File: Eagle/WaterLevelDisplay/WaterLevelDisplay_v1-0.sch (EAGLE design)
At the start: 17 parts, among them J12 POWER_JACKPTH_BREAD, J7 RJ45

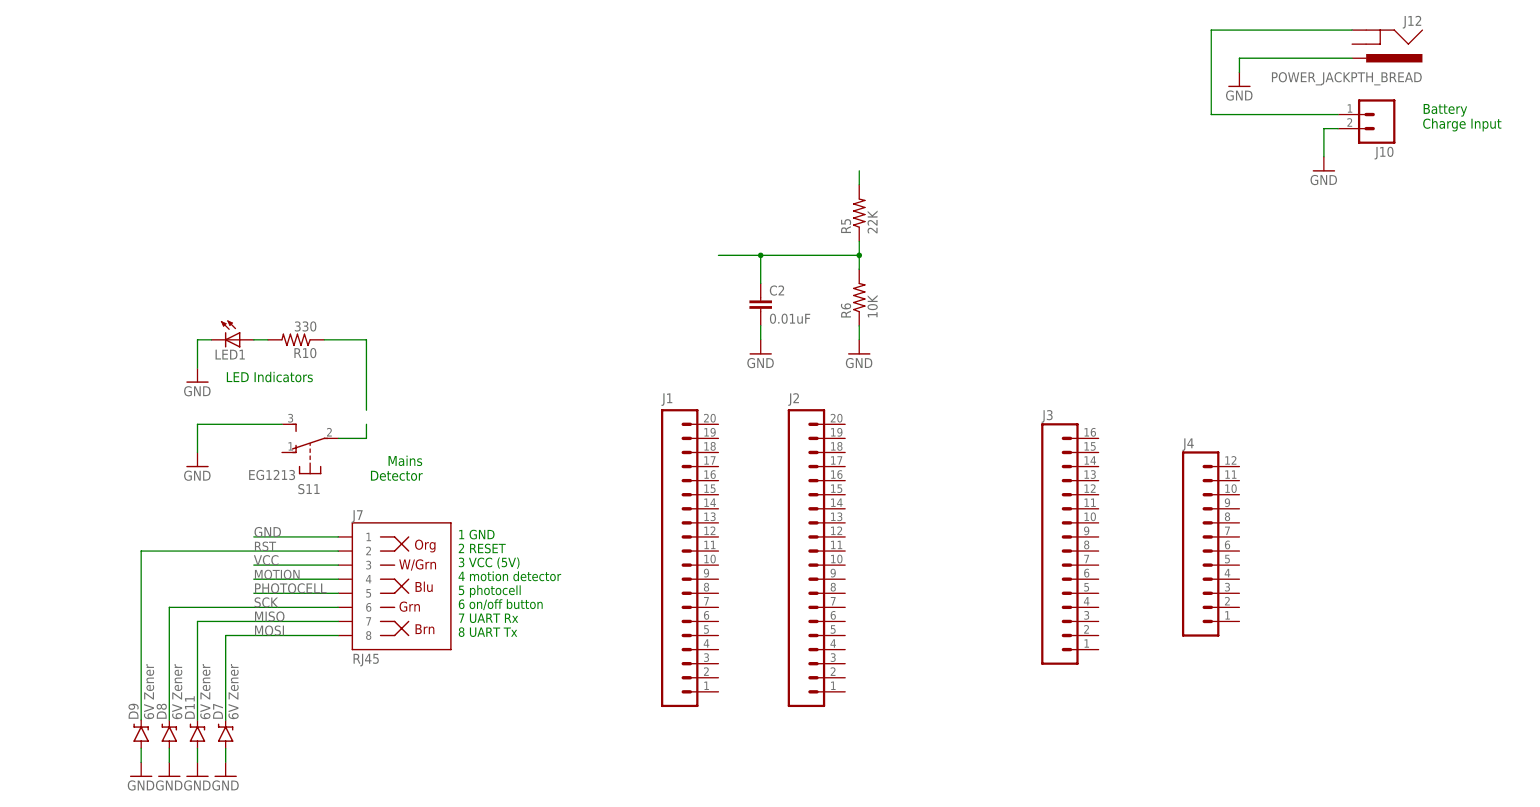
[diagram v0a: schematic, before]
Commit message: first round of layout
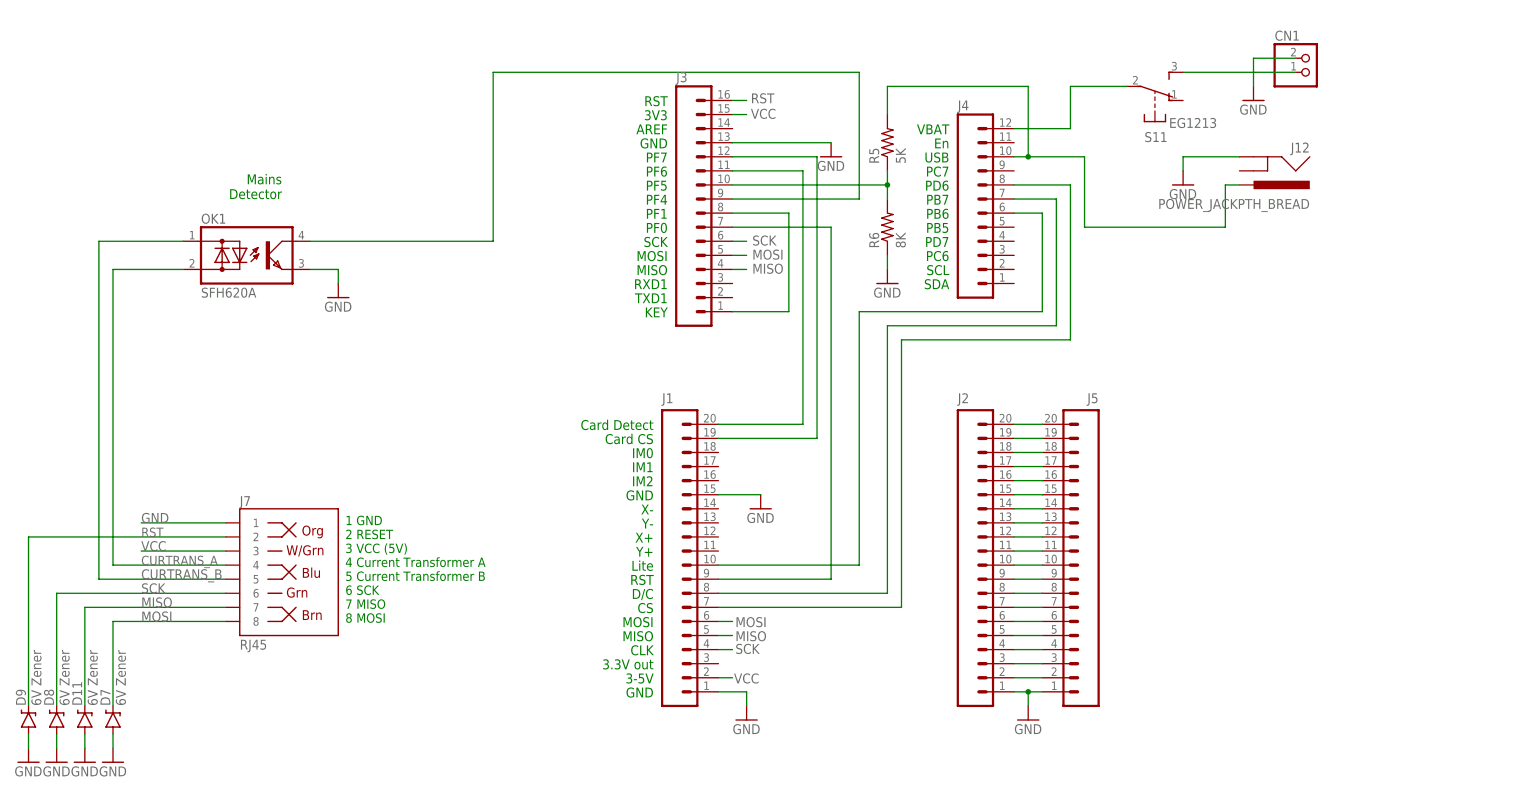
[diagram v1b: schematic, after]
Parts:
- removed C2: 0.01uF, SparkFun-Passives:CAPPTH1
- removed J10: (no value), SparkFun-Connectors:M02PTH
- removed LED1: (no value), adafruit:LED5MM
- removed R10: 330, resistor:R-US_0204/5
- added CN1: (no value), adafruit:JST_2PIN-SMT-RA
- added J5: (no value), SparkFun-Connectors:M20NOSILK
- added OK1: SFH620A, optocoupler:SFH620A
- R5: value 22K -> 5K
- R6: value 10K -> 8K
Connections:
- removed net MOTION: J7.4
- removed net N$6: C2.1, R5.1, R6.2
- removed net PHOTOCELL: J7.5
- new net CURTRANS_A: J7.4, OK1.AC2
- new net CURTRANS_B: J7.5, OK1.AC1
- new net N$10: J2.8, J5.8
- new net N$11: J2.9, J5.9
- new net N$12: J2.10, J5.10
- new net N$13: J2.11, J5.11
- new net N$14: J2.12, J5.12
- new net N$16: J2.13, J5.13
- new net N$19: J2.14, J5.14
- new net N$2: J2.2, J5.2
- new net N$20: J2.15, J5.15
- new net N$21: J2.16, J5.16
- new net N$22: J2.17, J5.17
- new net N$23: J2.18, J5.18
- new net N$24: J2.19, J5.19
- new net N$25: J2.20, J5.20
- new net N$27: J1.8, J4.7
- new net N$28: J1.19, J3.12
- new net N$29: J1.20, J3.11
- new net N$3: J2.3, J5.3
- new net N$30: J1.10, J4.6
- new net N$31: J3.9, OK1.C
- new net N$32: J1.7, J4.8
- new net N$33: J1.9, J3.7
- new net N$4: J2.4, J5.4
- new net N$5: J2.5, J5.5
- new net N$7: J2.6, J5.6
- new net N$8: J2.7, J5.7
- net GND: now also CN1.1, J1.1, J1.15, J12.GND, J2.1, J3.13, J5.1, OK1.E; no longer C2.2, J10.2, J12.PWR, LED1.C, S11.S
- net MISO: now also J1.5, J3.4
- net MOSI: now also J1.6, J3.5
- net N$1: now also CN1.2, S11.S; no longer LED1.A, R10.2
- net N$15: now also J3.1, J3.8; no longer R10.1
- net N$17: now also J12.PWR, J4.10, R5.2; no longer J10.1, J12.GND
- net N$18: now also J3.10, R5.1, R6.2; no longer R5.2
- net N$9: now also J4.12
- net RST: now also J3.16
- net SCK: now also J1.4, J3.6
- net VCC: now also J1.2, J3.15
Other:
- note added: "1 GND 2 RESET 3 VCC (5V) 4 Current Transformer A 5 Current Transformer B 6 SCK 7 MISO 8 MOSI"
- note added: "3-5V"
- note added: "3.3V out"
- note added: "3V3"
- note added: "AREF"
- note added: "CLK"
- note added: "CS"
- note added: "Card CS"
- note added: "Card Detect"
- note added: "D/C"
- note added: "En"
- note added: "GND"
- note added: "IM0"
- note added: "IM1"
- note added: "IM2"
- note added: "KEY"
- note added: "Lite"
- note added: "MISO"
- note added: "MOSI"
- note added: "PB5"
- note added: "PB6"
- note added: "PB7"
- note added: "PC6"
- note added: "PC7"
- note added: "PD6"
- note added: "PD7"
- note added: "PF0"
- note added: "PF1"
- note added: "PF4"
- note added: "PF5"
- note added: "PF6"
- note added: "PF7"
- note added: "RST"
- note added: "RXD1"
- note added: "SCK"
- note added: "SCL"
- note added: "SDA"
- note added: "TXD1"
- note added: "USB"
- note added: "VBAT"
- note added: "X+"
- note added: "X-"
- note added: "Y+"
- note added: "Y-"
- note removed: "1 GND 2 RESET 3 VCC (5V) 4 motion detector 5 photocell 6 on/off button 7 UART Rx 8 UART Tx"
- note removed: "Battery Charge Input"
- note removed: "LED Indicators"
- moved on the sheet: D11, D7, D8, D9, J12, J2, J3, J4, J7, R5, R6, S11
